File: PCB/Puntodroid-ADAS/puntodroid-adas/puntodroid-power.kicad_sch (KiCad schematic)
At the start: 13 parts, among them U8 MP1584-Step-Down, U9 AMS1117

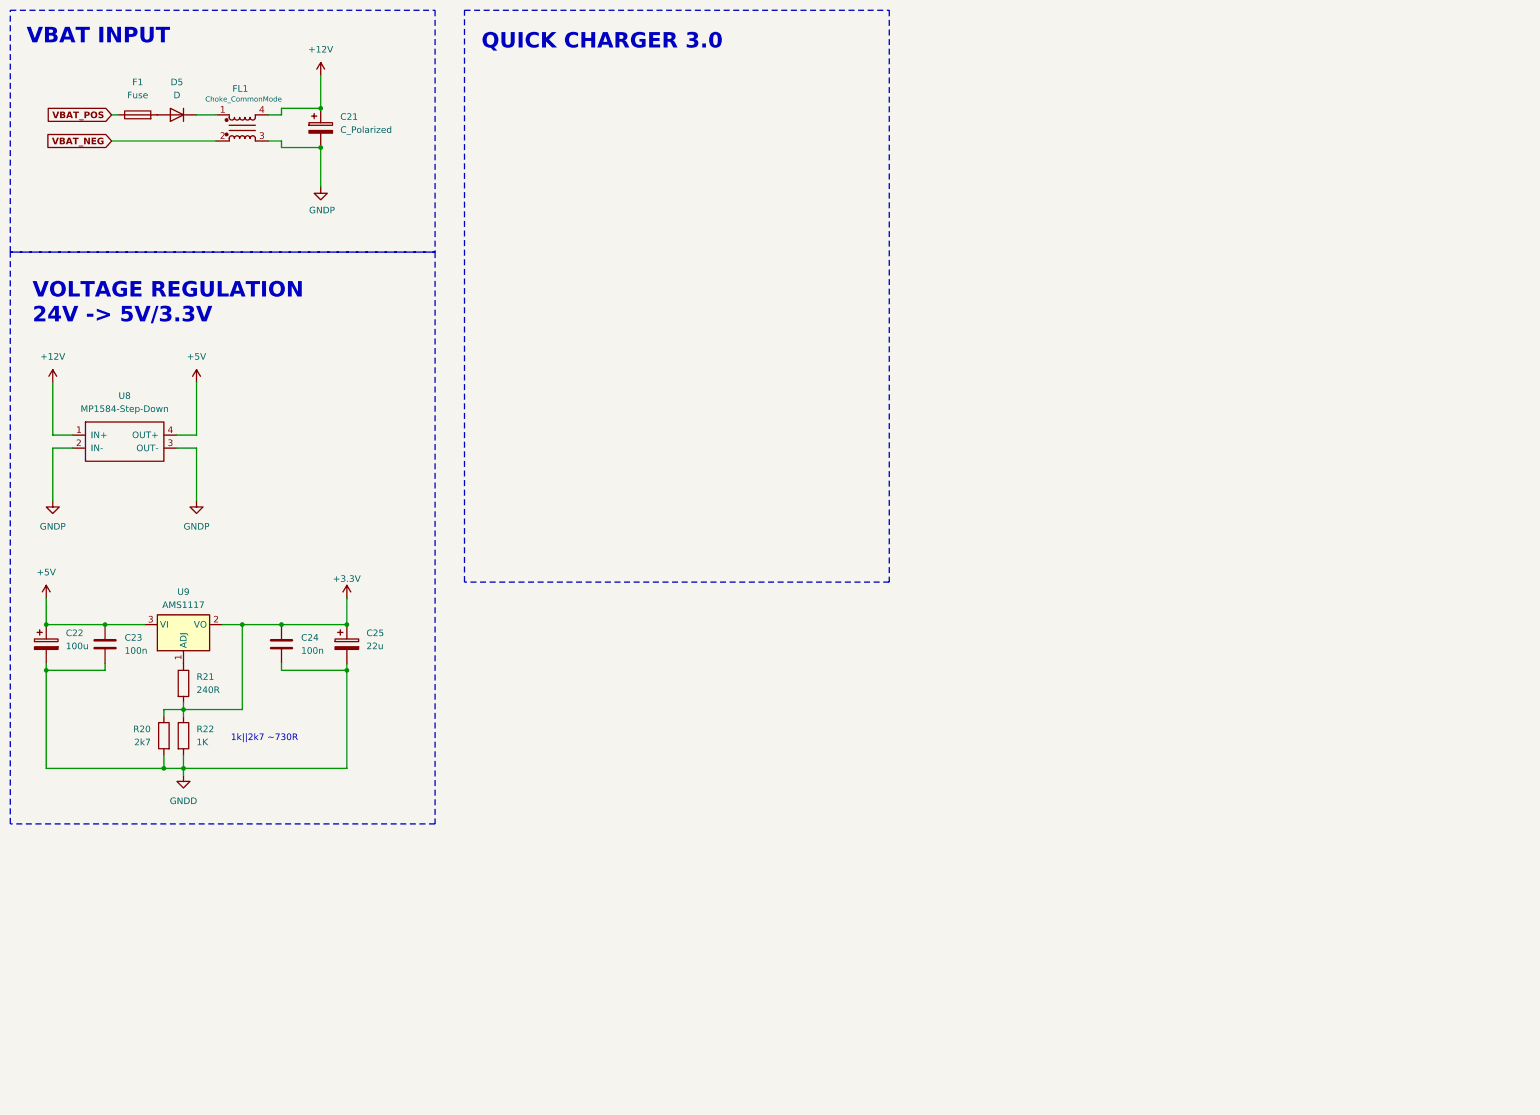
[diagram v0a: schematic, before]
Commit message: update puntodroid schematic stm32
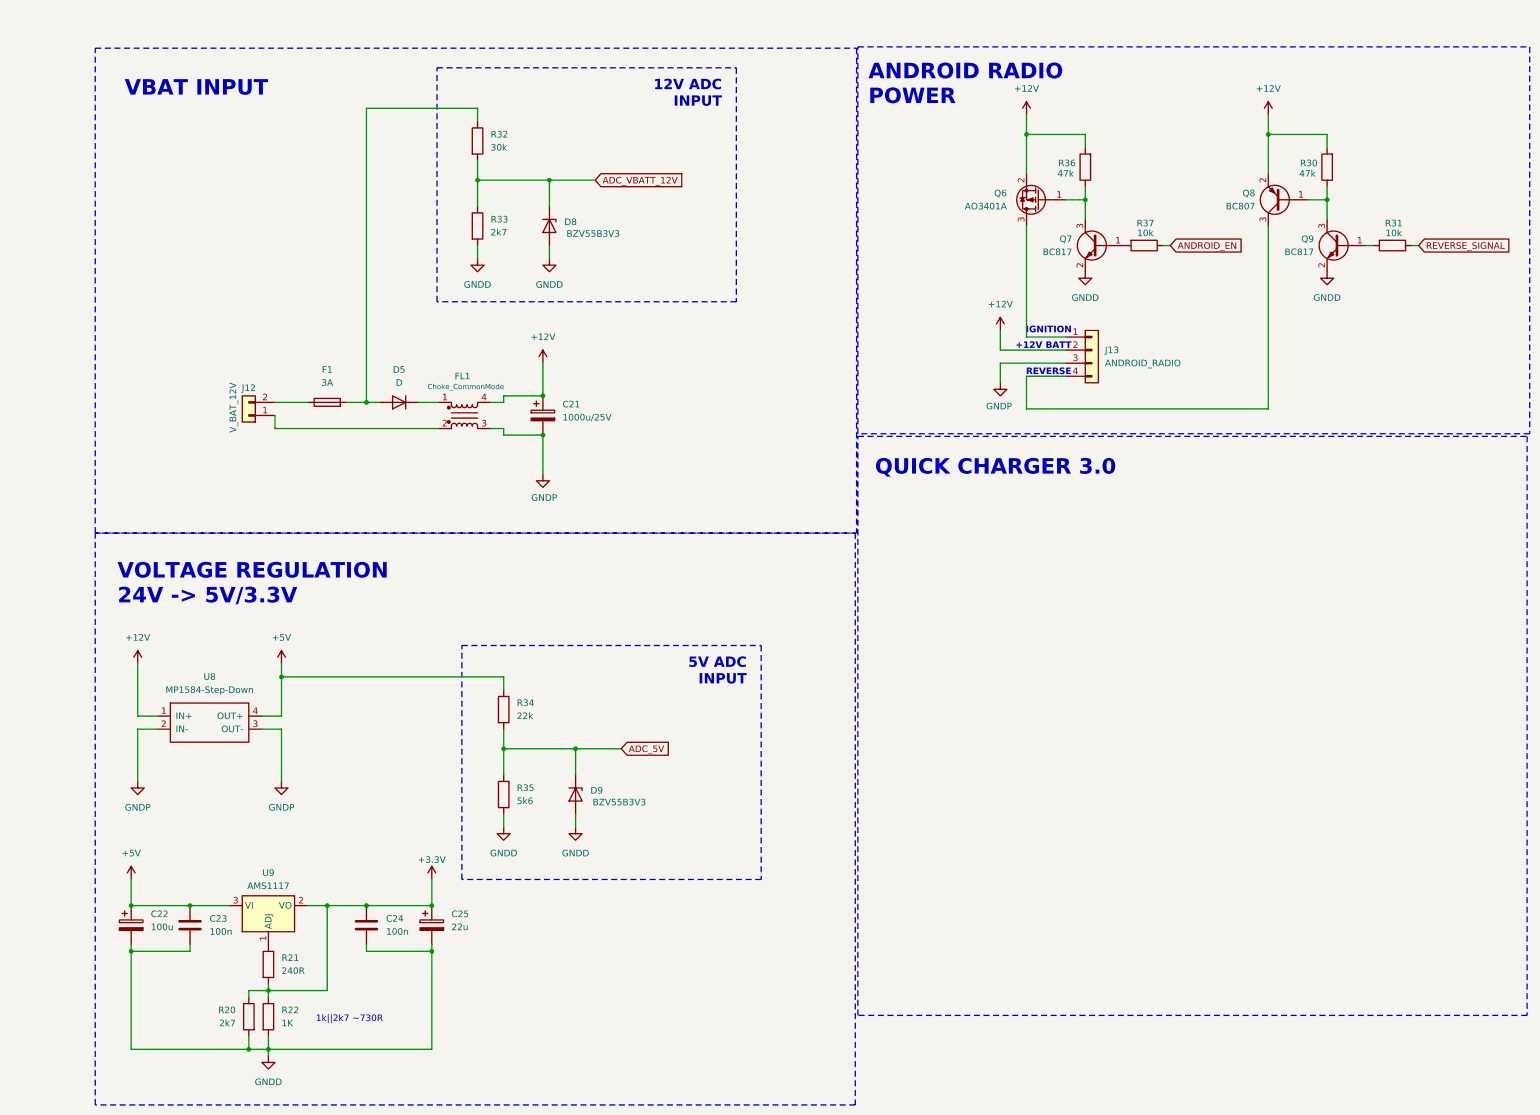
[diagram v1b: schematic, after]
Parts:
- added D8, D9: BZV55B3V3, Diode_SMD:D_MiniMELF, symbol Diode:BZV55B5V6
- added J12: V_BAT_12V, symbol Connector_Generic:Conn_01x02
- added J13: ANDROID_RADIO, symbol Connector_Generic:Conn_01x04
- added Q6: AO3401A, Package_TO_SOT_SMD:SOT-23, symbol Transistor_FET:AO3401A
- added Q7, Q9: BC817, Package_TO_SOT_SMD:SOT-23, symbol Transistor_BJT:BC817
- added Q8: BC807, Package_TO_SOT_SMD:SOT-23, symbol Transistor_BJT:BC807
- added R30, R36: 47k, symbol Device:R
- added R31, R37: 10k, symbol Device:R
- added R32: 30k, Resistor_SMD:R_0805_2012Metric_Pad1.20x1.40mm_HandSolder, symbol Device:R
- added R33: 2k7, Resistor_SMD:R_0805_2012Metric_Pad1.20x1.40mm_HandSolder, symbol Device:R
- added R34: 22k, Resistor_SMD:R_0805_2012Metric_Pad1.20x1.40mm_HandSolder, symbol Device:R
- added R35: 5k6, Resistor_SMD:R_0805_2012Metric_Pad1.20x1.40mm_HandSolder, symbol Device:R
- C21: value C_Polarized -> 1000u/25V
- F1: value Fuse -> 3A
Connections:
- net +12V: now also J13.2 (Pin_2), Q6.2 (S), Q8.2 (E), R30.2, R36.2
- net +5V: now also R34.1
- net GNDD: now also D8.2 (A), D9.2 (A), Q7.2 (E), Q9.2 (E), R33.2, R35.2
- net GNDP: now also J13.3 (Pin_3)
- net at D5.2 (A), F1.2: now also R32.1
- net VBAT_NEG: no longer names the net of FL1.2
- net VBAT_NEG: now also J12.1 (Pin_1)
- net VBAT_POS: no longer names the net of F1.1
- net VBAT_POS: now also J12.2 (Pin_2)
- new net: Q6.1 (G), Q7.3 (C), R36.1
- new net: J13.1 (Pin_1), Q6.3 (D)
- new net: J13.4 (Pin_4), Q8.3 (C)
- new net: Q7.1 (B), R37.2
- new net: Q9.1 (B), R31.2
- new net: Q8.1 (B), Q9.3 (C), R30.1
- new net ADC_5V: D9.1 (K), R34.2, R35.1
- new net ADC_VBATT_12V: D8.1 (K), R32.2, R33.1
- new net ANDROID_EN: R37.1
- new net REVERSE_SIGNAL: R31.1
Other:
- note added: "+12V BATT"
- note added: "12V ADC INPUT"
- note added: "5V ADC INPUT"
- note added: "ANDROID RADIO POWER"
- note added: "IGNITION"
- note added: "REVERSE"
- moved on the sheet: C21, C22, C23, C24, C25, D5, F1, FL1, R20, R21, R22, U8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
